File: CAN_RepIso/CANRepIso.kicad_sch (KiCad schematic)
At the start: 42 parts, among them U6 SN65HVD230, U7 PLACEHOLDER ISOLATOR, U8 SN65HVD230, U9 ADuM120N

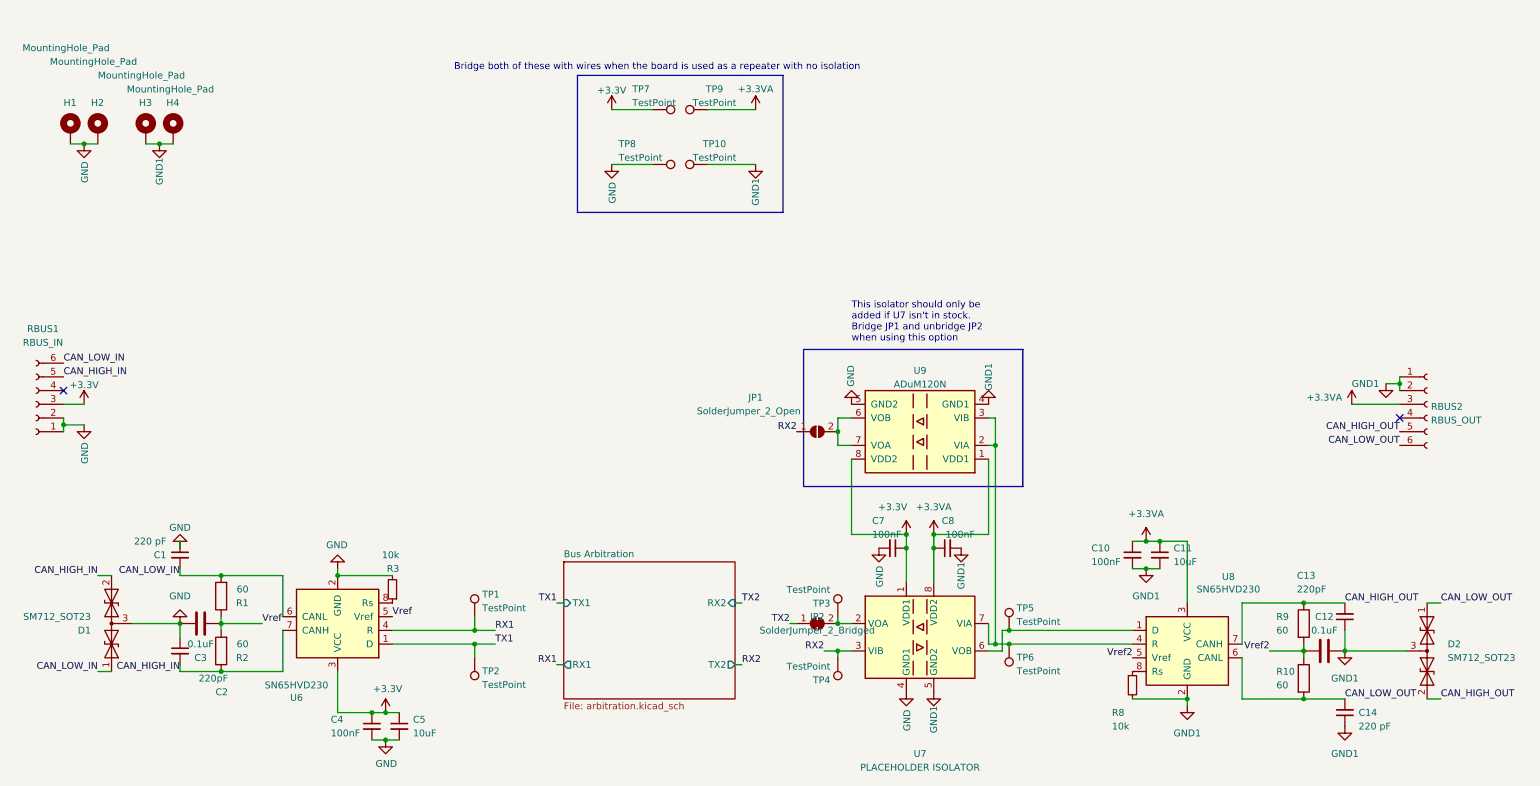
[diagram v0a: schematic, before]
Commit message: v2 finished pre-review
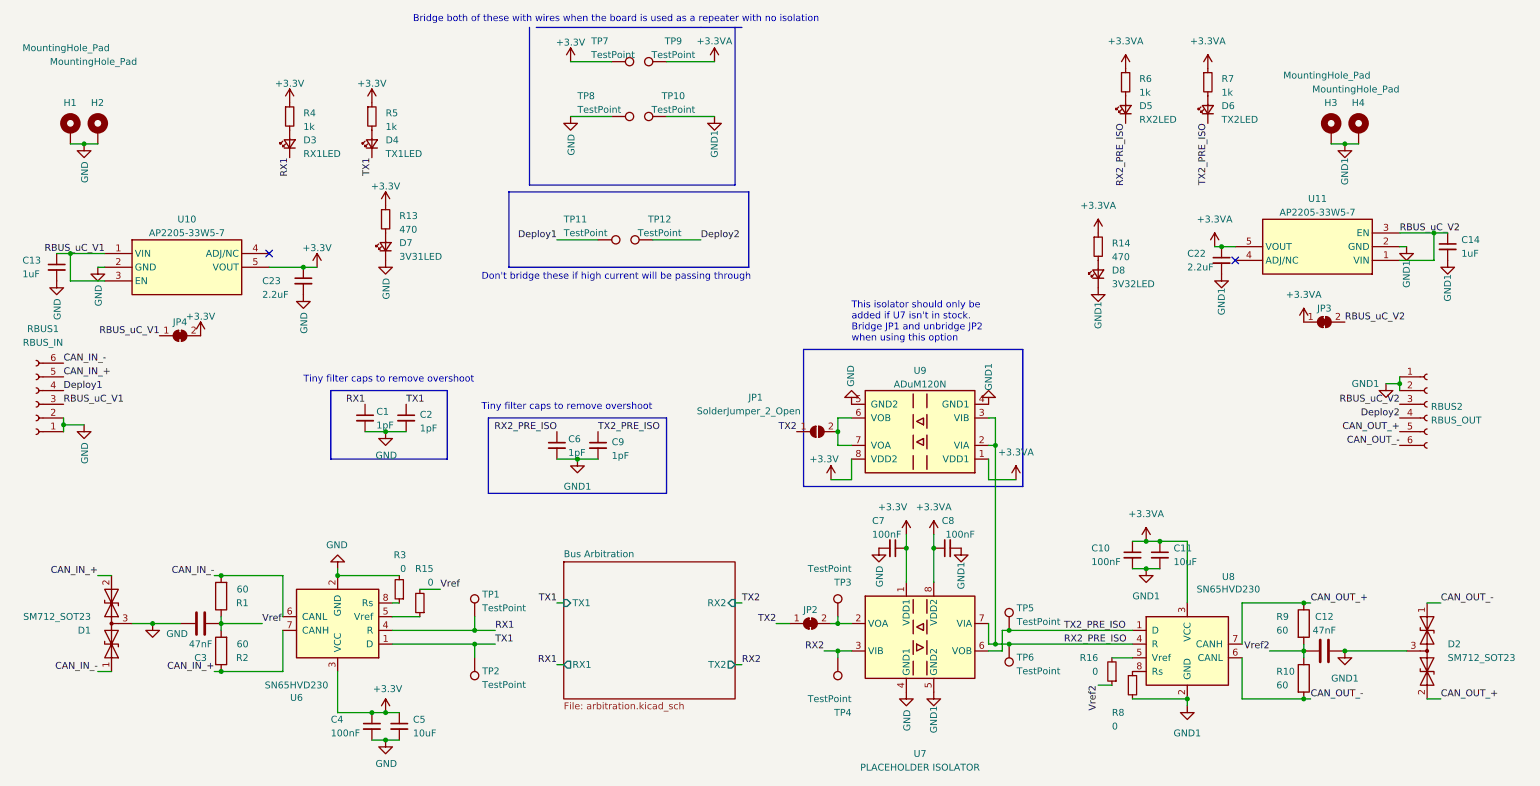
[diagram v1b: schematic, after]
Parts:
- added C22, C23: 2.2uF, Capacitor_SMD:C_0402_1005Metric, symbol Device:C_Small
- added C6, C9: 1pF, Capacitor_SMD:C_0402_1005Metric, symbol Device:C_Small
- added D3: RX1LED, LED_SMD:LED_0402_1005Metric, symbol Device:LED_Small
- added D4: TX1LED, LED_SMD:LED_0402_1005Metric, symbol Device:LED_Small
- added D5: RX2LED, LED_SMD:LED_0402_1005Metric, symbol Device:LED_Small
- added D6: TX2LED, LED_SMD:LED_0402_1005Metric, symbol Device:LED_Small
- added D7: 3V31LED, LED_SMD:LED_0402_1005Metric, symbol Device:LED_Small
- added D8: 3V32LED, LED_SMD:LED_0402_1005Metric, symbol Device:LED_Small
- added JP3, JP4: SolderJumper_2_Bridged, Jumper:SolderJumper-2_P1.3mm_Bridged_RoundedPad1.0x1.5mm, symbol Jumper:SolderJumper_2_Bridged
- added R13, R14: 470, Resistor_SMD:R_0402_1005Metric, symbol Device:R_Small
- added R15, R16: 0, Resistor_SMD:R_0402_1005Metric, symbol Device:R_Small
- added R4, R5, R6, R7: 1k, Resistor_SMD:R_0402_1005Metric, symbol Device:R_Small
- added TP11, TP12: TestPoint, Connector_PinHeader_2.54mm:PinHeader_1x01_P2.54mm_Vertical, symbol Connector:TestPoint
- added U10, U11: AP2205-33W5-7, iclr:SOT95P282X145-5N, symbol iclr:AP2205-W5-7
- C1: value 220 pF -> 1pF; footprint Capacitor_SMD:C_0603_1608Metric -> Capacitor_SMD:C_0402_1005Metric
- C10, C11, C4, C5, C7, C8: footprint Capacitor_SMD:C_0603_1608Metric -> Capacitor_SMD:C_0402_1005Metric
- C12, C3: value 0.1uF -> 47nF; footprint Capacitor_SMD:C_0603_1608Metric -> Capacitor_SMD:C_0402_1005Metric
- C13: value 220pF -> 1uF; footprint Capacitor_SMD:C_0603_1608Metric -> Capacitor_SMD:C_0402_1005Metric
- C14: value 220 pF -> 1uF; footprint Capacitor_SMD:C_0603_1608Metric -> Capacitor_SMD:C_0402_1005Metric
- C2: value 220pF -> 1pF; footprint Capacitor_SMD:C_0603_1608Metric -> Capacitor_SMD:C_0402_1005Metric
- R1, R10, R2, R9: footprint Resistor_SMD:R_0805_2012Metric -> Resistor_SMD:R_0603_1608Metric
- R3, R8: value 10k -> 0
- RBUS1, RBUS2: footprint Connector_Molex:Molex_Mini-Fit_Jr_5566-06A_2x03_P4.20mm_Vertical -> Connector_Molex:Molex_Mini-Fit_Jr_5569-06A2_2x03_P4.20mm_Horizontal
- TP1, TP2, TP3, TP4, TP5, TP6: footprint TestPoint:TestPoint_Pad_D1.5mm -> TestPoint:TestPoint_Pad_D1.0mm
- TP10, TP7, TP8, TP9: footprint TestPoint:TestPoint_Pad_D2.0mm -> Connector_PinHeader_2.54mm:PinHeader_1x01_P2.54mm_Vertical
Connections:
- net +3.3VA: now also C22.1, JP3.1 (A), R14.1, R6.1, R7.1, U11.5 (VOUT); no longer RBUS2.3 (Pin_3)
- net +3V3: now also C23.1, JP4.2 (B), R13.1, R4.1, R5.1, U10.5 (VOUT); no longer RBUS1.3 (Pin_3)
- net GND: now also C1.2, C13.2, C2.2, C23.2, D7.1 (K), U10.2 (GND); no longer C1.1, C2.1
- net GND1: now also C14.2, C22.2, C6.2, C9.2, D8.1 (K), U11.2 (GND); no longer C13.1, C14.1
- net RX1: now also C1.1, D3.1 (K)
- net RX2: no longer JP1.1 (A)
- net TX1: now also C2.1, D4.1 (K)
- net TX2: now also JP1.1 (A)
- net Vref: now also R15.2; no longer U6.5 (Vref)
- net Vref2: now also R16.1; no longer U8.5 (Vref)
- net TX2_PRE_ISO: now reaches TP5.1, U7.6 (VOB), U8.1 (D)
- net TX2_PRE_ISO: now also C9.1, D6.1 (K)
- net RX2_PRE_ISO: now reaches TP6.1, U7.7 (VIA), U8.4 (R), U9.2 (VIA), U9.3 (VIB)
- net RX2_PRE_ISO: now also C6.1, D5.1 (K)
- net Deploy1: now reaches RBUS1.4 (Pin_4)
- net Deploy1: now also TP11.1
- net Deploy2: now reaches RBUS2.4 (Pin_4)
- net Deploy2: now also TP12.1
- net CAN_HIGH_IN renamed CAN_IN_+
- net CAN_IN_+: no longer C2.2
- net CAN_HIGH_OUT renamed CAN_OUT_+
- net CAN_OUT_+: no longer C13.2
- net CAN_LOW_IN renamed CAN_IN_-
- net CAN_IN_-: no longer C1.2
- net CAN_LOW_OUT renamed CAN_OUT_-
- net CAN_OUT_-: no longer C14.2
- new net: D8.2 (A), R14.2
- new net: D3.2 (A), R4.2
- new net: R15.1, U6.5 (Vref)
- new net: D7.2 (A), R13.2
- new net: D4.2 (A), R5.2
- new net: R16.2, U8.5 (Vref)
- new net: D5.2 (A), R6.2
- new net: D6.2 (A), R7.2
- new net RBUS_uC_V1: C13.1, JP4.1 (A), RBUS1.3 (Pin_3), U10.1 (VIN), U10.3 (EN)
- new net RBUS_uC_V2: C14.1, JP3.2 (B), RBUS2.3 (Pin_3), U11.1 (VIN), U11.3 (EN)
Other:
- note added: "Don't bridge these if high current will be passing through"
- note added: "Tiny filter caps to remove overshoot"
- company: (none) -> ICLR
- title: (none) -> CAN Repeater and Isolator
- moved on the sheet: H3, H4, JP2, R3, TP10, TP7, TP8, TP9
